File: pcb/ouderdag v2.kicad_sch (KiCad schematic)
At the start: 18 parts, among them J1 Conn_01x05_Pin, J2 Conn_01x05_Pin, J3 Conn_01x05_Socket, J4 Conn_01x05_Socket, J5 Conn_01x06_Pin, SW1 SW_Push, U1 ATtiny85

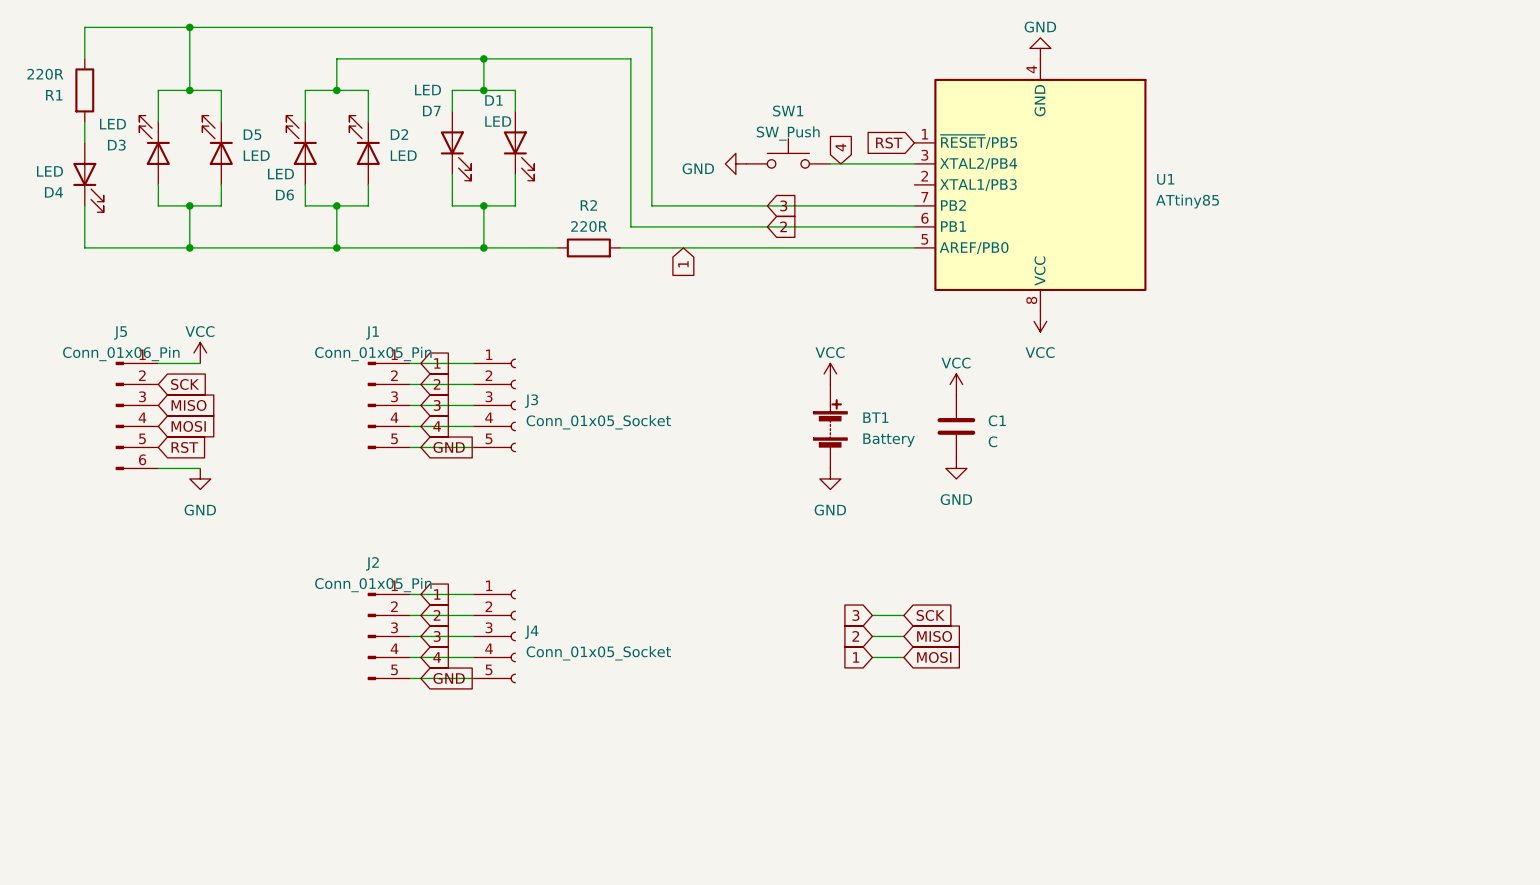
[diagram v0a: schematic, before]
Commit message: updated code and pcb
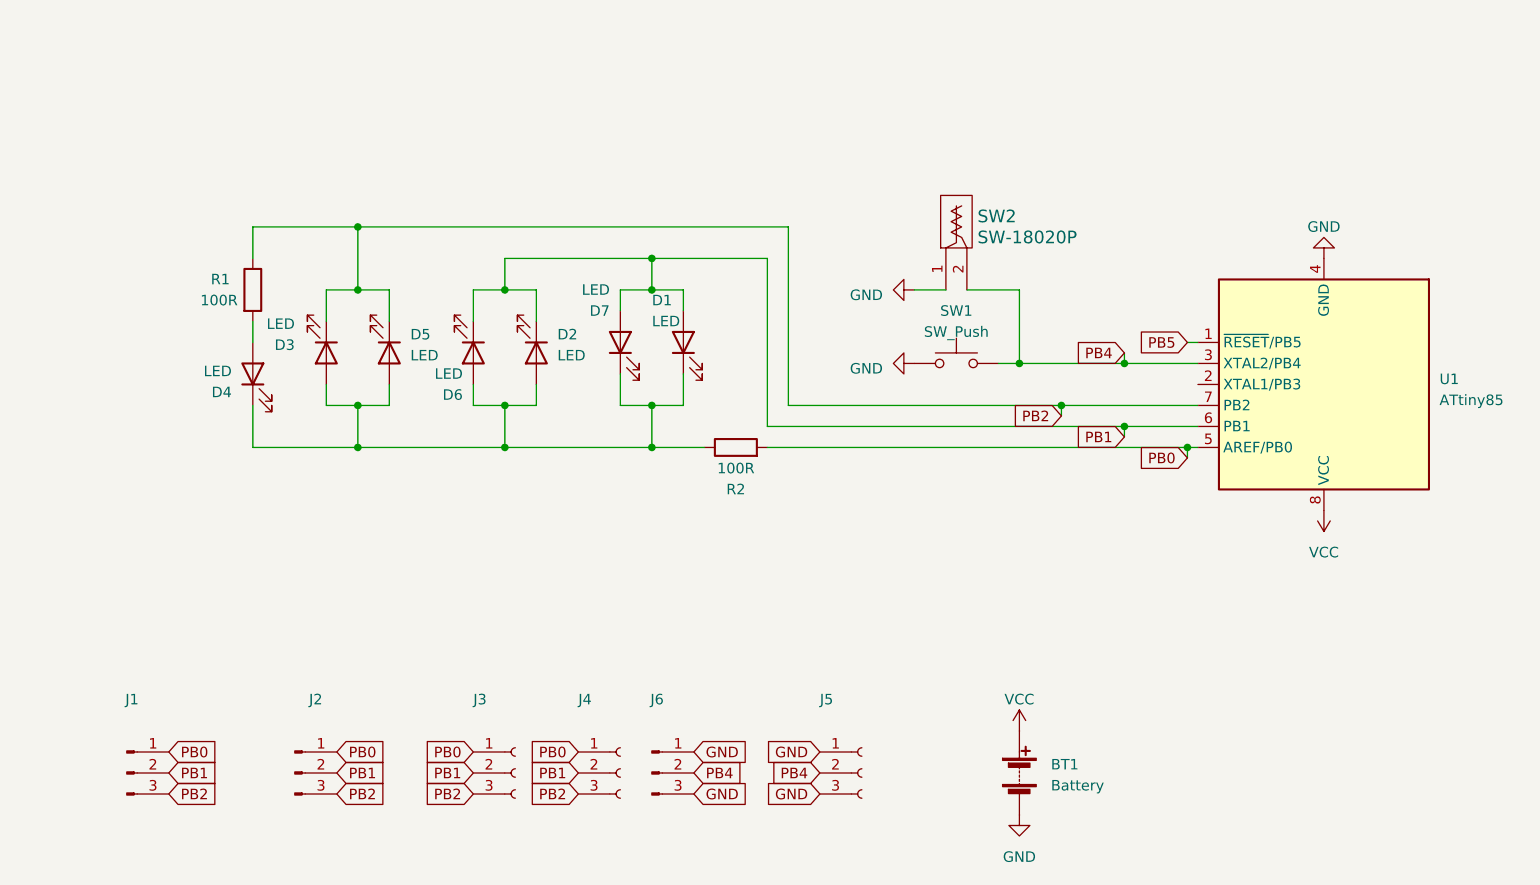
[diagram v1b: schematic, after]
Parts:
- removed C1: C, Capacitor_THT:CP_Radial_D8.0mm_P3.50mm, symbol Device:C
- removed J5: Conn_01x06_Pin, Connector_PinHeader_2.54mm:PinHeader_1x06_P2.54mm_Vertical, symbol Connector:Conn_01x06_Pin
- added J5: Conn_01x03_Socket, Connector_PinSocket_2.54mm:PinSocket_1x03_P2.54mm_Vertical, symbol Connector:Conn_01x03_Socket
- added J6: Conn_01x03_Pin, Connector_PinHeader_2.54mm:PinHeader_1x03_P2.54mm_Vertical, symbol Connector:Conn_01x03_Pin
- added SW2: SW-18020P, lib:SW-18020P, symbol rur:SW-18020P
- D1, D2, D3, D4, D5, D6, D7: footprint LED_THT:LED_D8.0mm -> LED_THT:LED_D10.0mm
- J1, J2: value Conn_01x05_Pin -> Conn_01x03_Pin; footprint Connector_PinHeader_2.54mm:PinHeader_1x05_P2.54mm_Vertical -> Connector_PinHeader_2.54mm:PinHeader_1x03_P2.54mm_Vertical; symbol Connector:Conn_01x05_Pin -> Connector:Conn_01x03_Pin
- J3, J4: value Conn_01x05_Socket -> Conn_01x03_Socket; footprint Connector_PinSocket_2.54mm:PinSocket_1x05_P2.54mm_Vertical -> Connector_PinSocket_2.54mm:PinSocket_1x03_P2.54mm_Vertical; symbol Connector:Conn_01x05_Socket -> Connector:Conn_01x03_Socket
- R1, R2: value 220R -> 100R
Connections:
- net GND: now also J5.1 (Pin_1), J5.3 (Pin_3), J6.1 (Pin_1), J6.3 (Pin_3), SW2.1; no longer J1.5 (Pin_5), J2.5 (Pin_5), J3.5 (Pin_5), J4.5 (Pin_5)
- net 1 renamed PB0
- net 2 renamed PB1
- net 3 renamed PB2
- removed net 4: J1.4 (Pin_4), J2.4 (Pin_4), J3.4 (Pin_4), J4.4 (Pin_4), SW1.2, U1.3 (XTAL2/PB4)
- net RST renamed PB5
- new net PB4: J5.2 (Pin_2), J6.2 (Pin_2), SW1.2, SW2.2, U1.3 (XTAL2/PB4)
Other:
- moved on the sheet: BT1, D1, D2, D3, D4, D5, D6, D7, R1, R2, SW1, U1
